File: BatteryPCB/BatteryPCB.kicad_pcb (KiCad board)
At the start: 2 copper layers, 68.6 x 53.3 mm, 22 parts, among them J1 Conn_01x01, J2 Conn_01x01, J3 Conn_01x01, J4 Conn_01x01_Socket, SW1 ANT11TFHQE, SW3 ANT11TFHQE, U1 LF50CV, U2 R05-100B, U3 R05-100B

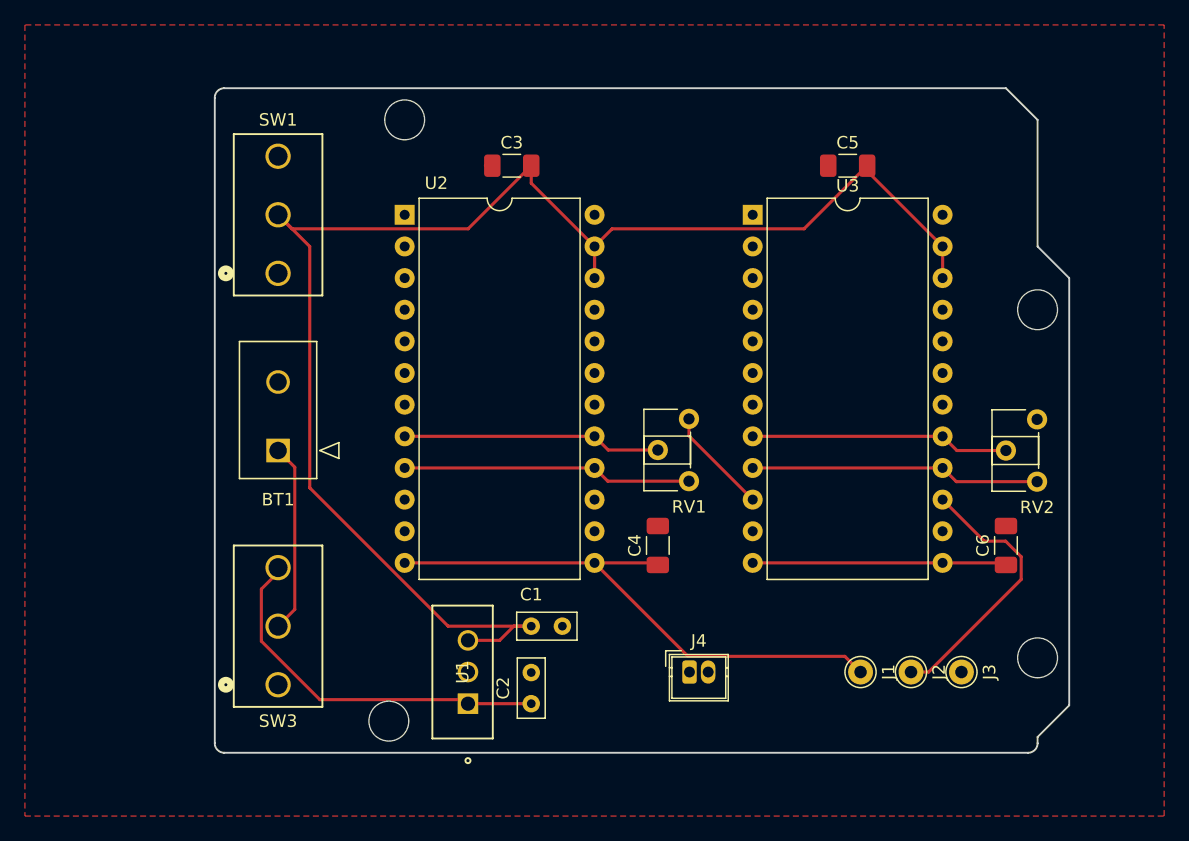
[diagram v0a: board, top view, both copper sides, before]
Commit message: 2nd Update from 3/29 comments
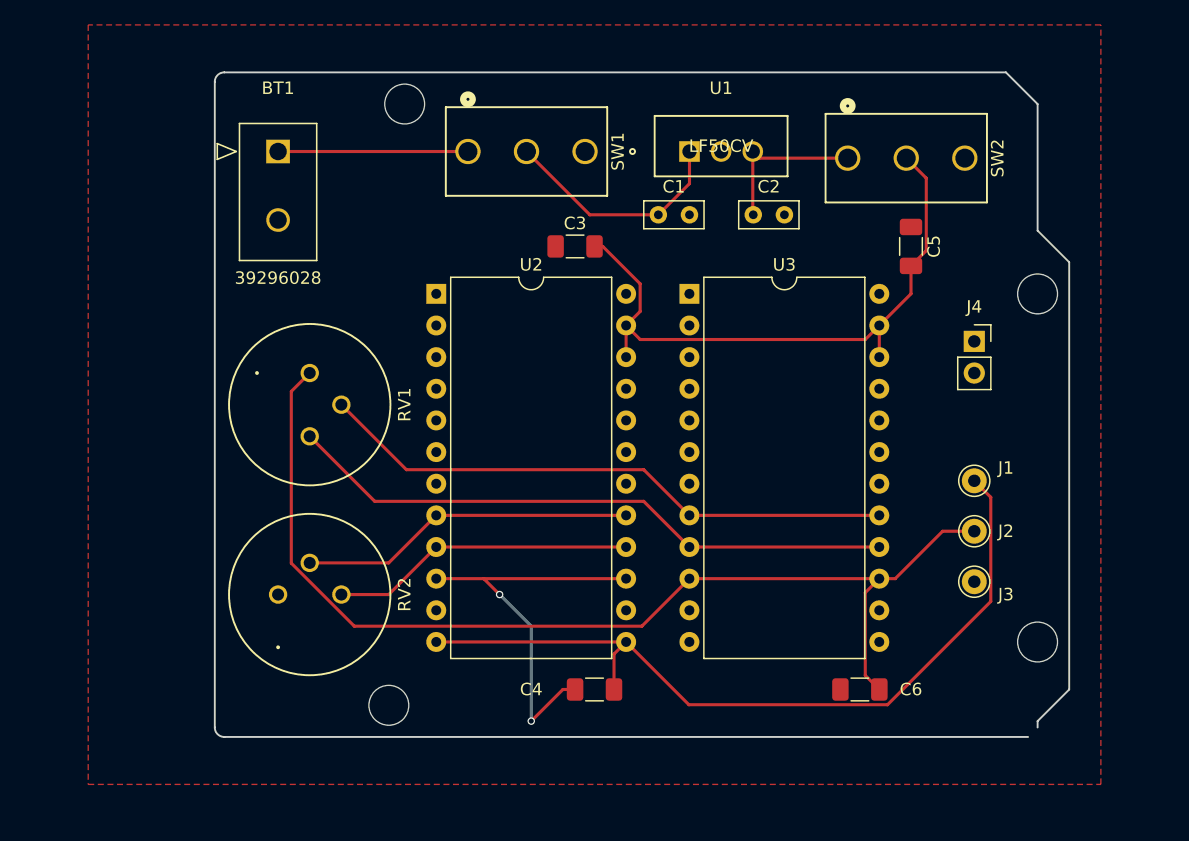
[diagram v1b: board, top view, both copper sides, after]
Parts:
- removed SW3: ANT11TFHQE, 100SP1T1B4M2QE:100SP1T1_EWI
- added SW2: ANT11TFHQE, 100SP1T1B4M2QE:100SP1T1_EWI, F.Cu at (150.8, 52.3)
- C1: value 0.1μF -> 0.33μF
- C2: value 0.33μF -> 0.1μF
- J4: footprint Connector_Wuerth:Wuerth_WR-WTB_64800211622_1x02_P1.50mm_Vertical -> Connector_PinSocket_2.54mm:PinSocket_1x02_P2.54mm_Vertical
- RV1, RV2: value 5kΩ -> 93PR5KLF; footprint Potentiometer_THT:Potentiometer_ACP_CA6-H2,5_Horizontal -> 93PR5KL:RES3_93_TTE
- U1: footprint L7805CV:TO-220_STM -> LF50CV:LF50CV
- moved RV2 56.6 mm to (110.2, 87.3), turned to 0 degrees
- moved U1 47.8 mm to (138.1, 51.7), turned to 0 degrees
- moved C2 43.1 mm to (143.2, 56.8), turned to 0 degrees
- moved J4 35.0 mm to (161.0, 67.0)
- moved C1 34.6 mm to (135.6, 56.8)
- moved RV1 30.7 mm to (107.6, 74.6), turned to -90 degrees
- moved BT1 24.0 mm to (105.1, 51.7), turned to 0 degrees
- moved SW1 18.1 mm to (120.3, 51.7), turned to 90 degrees
- moved J1 17.9 mm to (161.0, 78.2), turned to 0 degrees
- moved C6 16.5 mm to (151.8, 94.9), turned to 180 degrees
- moved C4 12.6 mm to (130.5, 94.9), turned to 0 degrees
- moved J2 12.4 mm to (161.0, 82.2), turned to 0 degrees
- moved C3 8.23 mm to (128.9, 59.4)
- moved C5 8.23 mm to (155.9, 59.4), turned to -90 degrees
- moved U3 8.13 mm to (138.1, 63.2)
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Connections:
- C1 pad 1: +5V -> Net-(U1-IN)
- C2 pad 1: Net-(SW3A-C) -> +5V
- C3 pad 2: +5V -> Net-(C3-Pad2)
- C4 pad 1: HT -> GND
- C4 pad 2: GND -> HT
- C5 pad 2: +5V -> Net-(C3-Pad2)
- C6 pad 1: Net-(C6-Pad1) -> -VSW
- RV1 pad 2: Net-(U2-VADJ) -> Net-(RV1-Pad2)
- RV1 pad 3: GND -> -VSW
- RV2 pad 2: Net-(U3-VADJ) -> Net-(RV2-Pad2)
- SW1 pad 1: unconnected-(SW1A-A-Pad1) -> Net-(BT1-+)
- SW1 pad 2: +5V -> Net-(U1-IN)
- SW1 pad 3: GND -> (no net)
- U1 pad 1: Net-(SW3A-C) -> Net-(U1-IN)
- U2 pad 16: Net-(RV1-Pad1) -> Net-(RV2-Pad1)
- U2 pad 17: Net-(U2-VADJ) -> Net-(RV2-Pad2)
- U2 pad 22: +5V -> Net-(C3-Pad2)
- U2 pad 23: +5V -> Net-(C3-Pad2)
- U2 pad 8: Net-(U2-VADJ) -> Net-(RV2-Pad2)
- U2 pad 9: Net-(RV1-Pad1) -> Net-(RV2-Pad1)
- U3 pad 10: GND -> -VSW
- U3 pad 12: Net-(C6-Pad1) -> GND
- U3 pad 13: Net-(C6-Pad1) -> GND
- U3 pad 16: Net-(RV2-Pad1) -> Net-(RV1-Pad1)
- U3 pad 17: Net-(U3-VADJ) -> Net-(RV1-Pad2)
- U3 pad 22: +5V -> Net-(C3-Pad2)
- U3 pad 23: +5V -> Net-(C3-Pad2)
- U3 pad 8: Net-(U3-VADJ) -> Net-(RV1-Pad2)
- U3 pad 9: Net-(RV2-Pad1) -> Net-(RV1-Pad1)
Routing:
- net +5V: track 123.5 -> 12.9 mm
- net -VSW: track 21.5 -> 85.8 mm
- net Net-(C3-Pad2): track 0.00 -> 50.7 mm
- net Net-(RV1-Pad2): track 0.00 -> 46.9 mm
- net Net-(SW3A-C): track 29.8 -> 0.00 mm
- net Net-(RV2-Pad2): track 0.00 -> 27.0 mm
- net Net-(RV1-Pad1): track 23.3 -> 49.4 mm
- net GND: track 9.79 -> 32.8 mm, vias 0 -> 2
- net Net-(U3-VADJ): track 20.8 -> 0.00 mm
- net Net-(U2-VADJ): track 20.8 -> 0.00 mm
- net Net-(C6-Pad1): track 20.2 -> 0.00 mm
- net HT: track 45.4 -> 64.5 mm
- net Net-(U1-IN): track 0.00 -> 18.8 mm
- net Net-(RV2-Pad1): track 23.3 -> 24.4 mm
